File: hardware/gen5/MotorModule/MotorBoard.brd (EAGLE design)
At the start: 49.7 x 28.5 mm, 44 parts

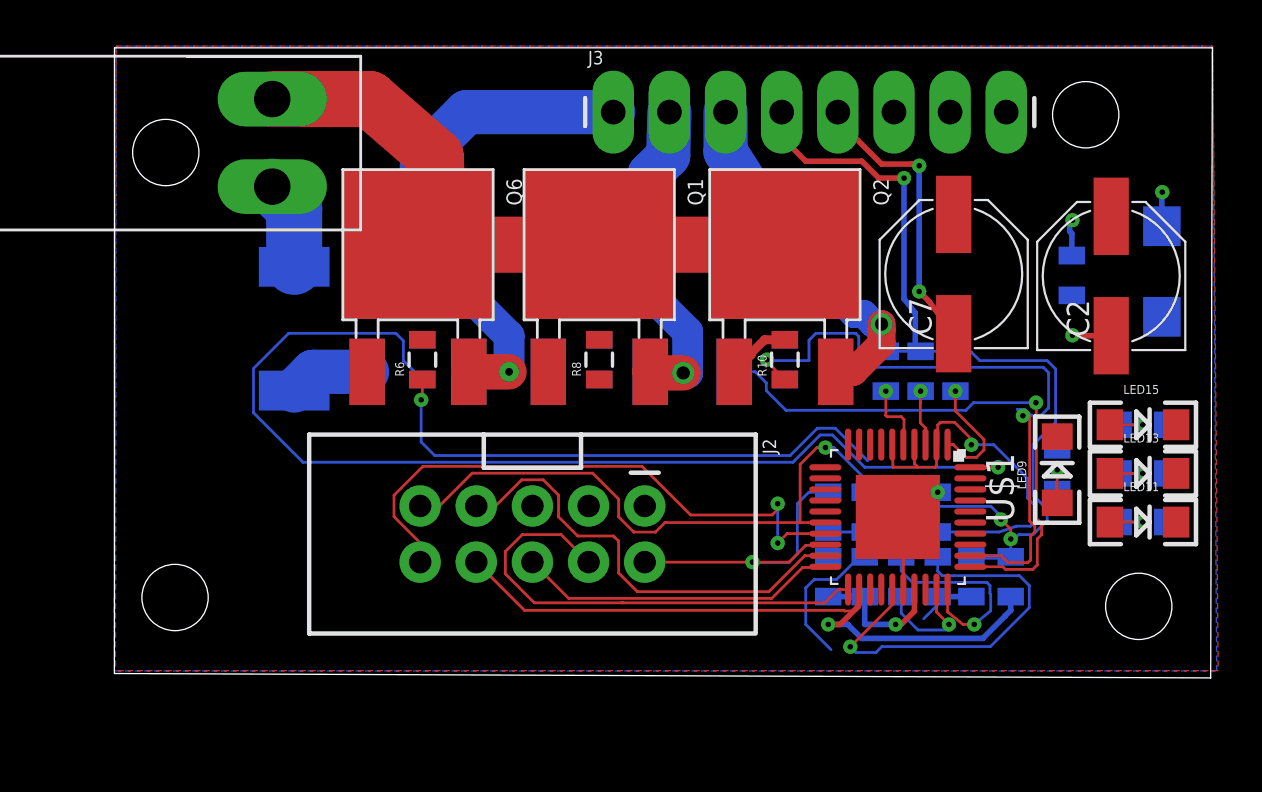
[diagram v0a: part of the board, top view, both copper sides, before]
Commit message: more routing nearly there
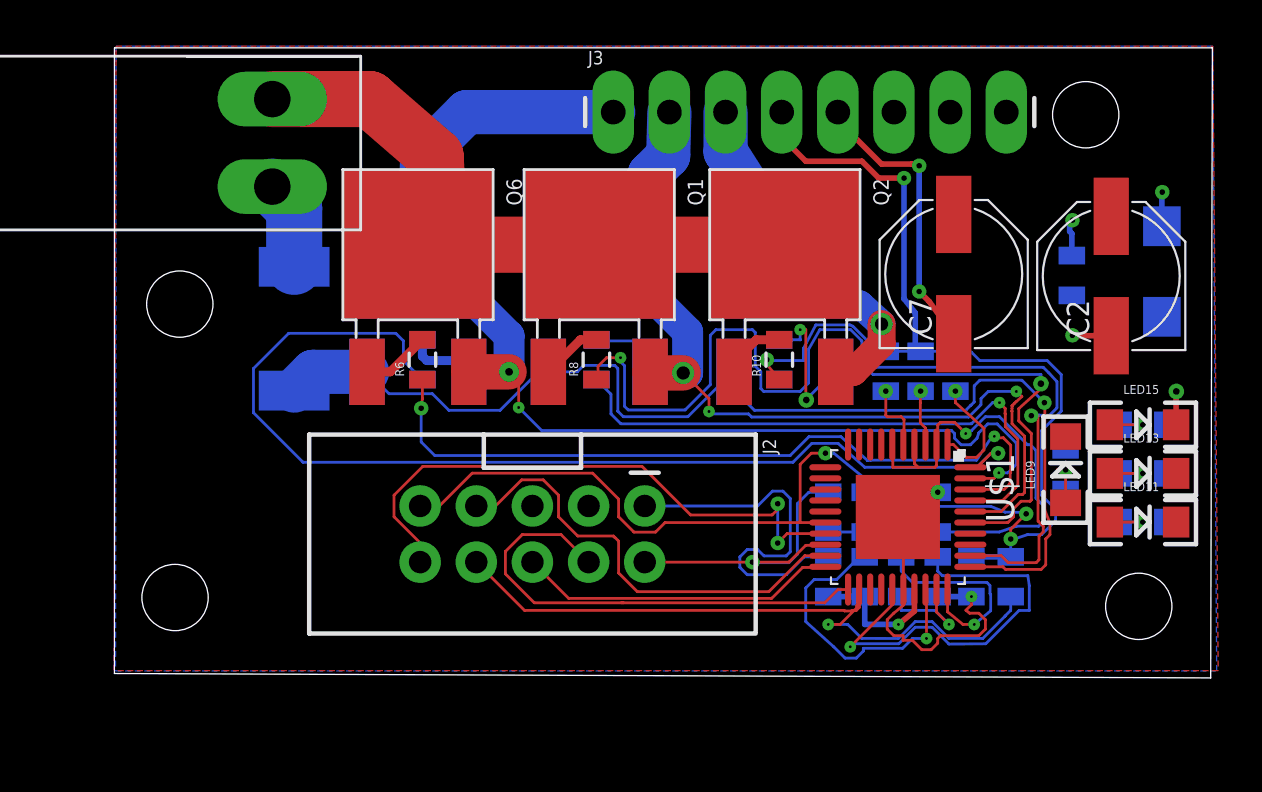
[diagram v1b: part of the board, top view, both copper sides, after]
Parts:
- moved LED9 0.38 mm to (54.3, 30.6)
- moved R1 0.38 mm to (54.3, 30.6)
- moved R10 0.25 mm to (41.3, 35.6)
- moved R14 0.25 mm to (41.3, 35.6)
- moved R13 0.13 mm to (33.1, 35.6)
- moved R8 0.13 mm to (33.1, 35.6)
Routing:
- net N$20: track 0.00 -> 42.1 mm, vias 0 -> 2
- net M1O1: track 22.7 -> 52.1 mm, vias 1 -> 3
- net GND: track 25.0 -> 52.4 mm, vias 4 -> 6
- net N$18: track 0.00 -> 26.5 mm, vias 0 -> 1
- net M1O2: track 13.6 -> 38.5 mm, vias 1 -> 3
- net O1: track 29.1 -> 53.3 mm
- net N$16: track 24.4 -> 35.0 mm, vias 1 -> 2
- net N$4: track 6.52 -> 13.6 mm, vias 0 -> 1
- net N$14: track 0.00 -> 6.99 mm, vias 0 -> 2
- net N$13: track 0.00 -> 3.84 mm
- net N$11: track 0.00 -> 3.13 mm
- net N$6: track 0.00 -> 3.10 mm
- net N$7: track 0.00 -> 2.77 mm
- net N$22: track 21.3 -> 23.2 mm
- net 5V: track 46.9 -> 48.6 mm
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
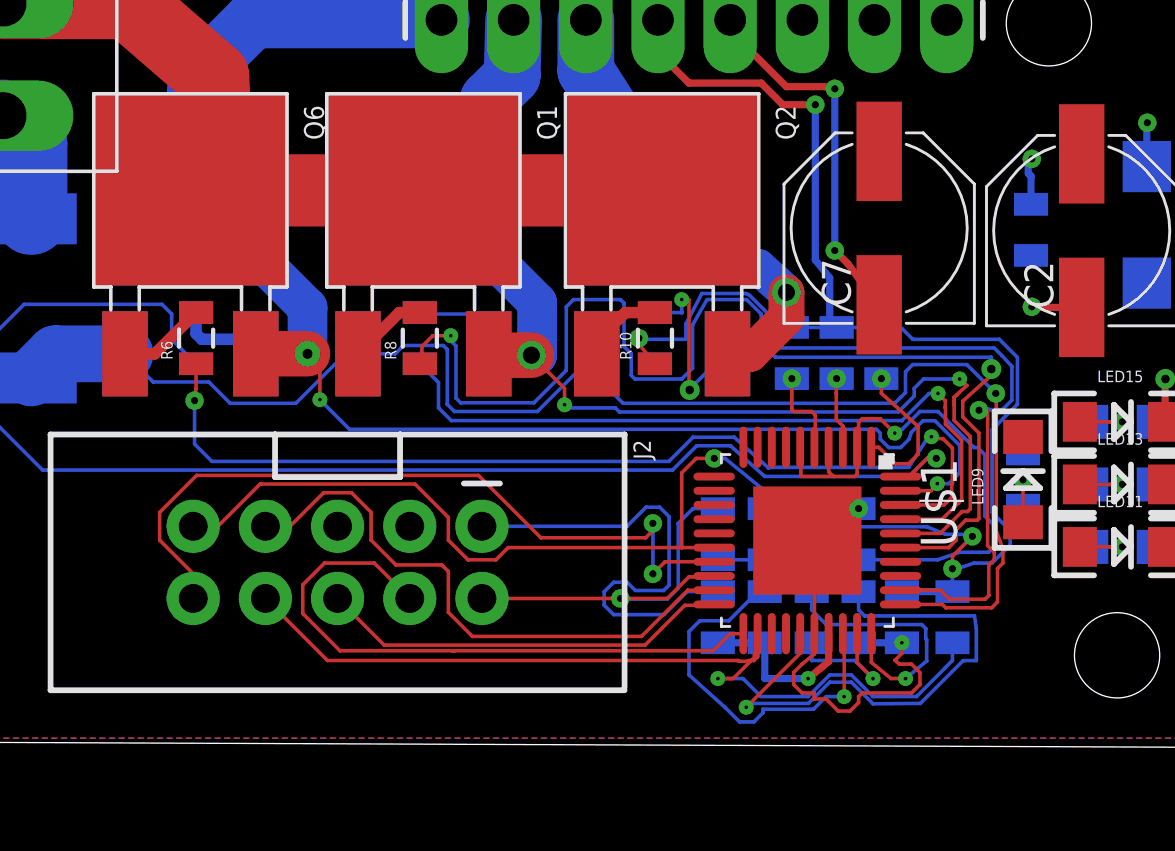
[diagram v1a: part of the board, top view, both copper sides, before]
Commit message: more routing
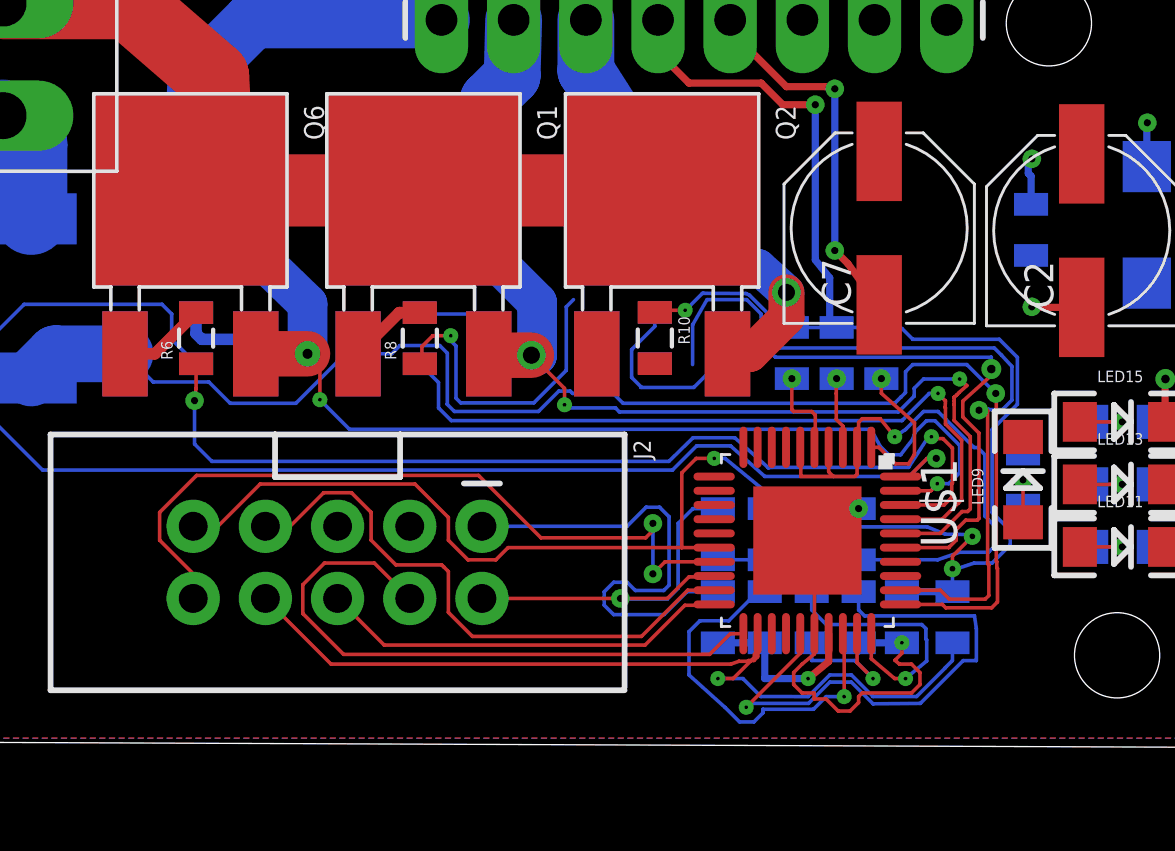
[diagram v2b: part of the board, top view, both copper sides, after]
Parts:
- turned R10 to 270 degrees
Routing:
- net N$20: track 42.1 -> 35.2 mm
- net N$10: track 2.84 -> 0.07 mm
- net N$21: track 29.9 -> 27.2 mm
- net O1: track 53.3 -> 50.7 mm
- net N$14: track 6.99 -> 6.65 mm, vias 2 -> 0
